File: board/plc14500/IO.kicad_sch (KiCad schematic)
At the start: 72 parts, among them U1 74HC14, U2 4051, U3 74HC14, U5 4099, U6 Arduino Nano

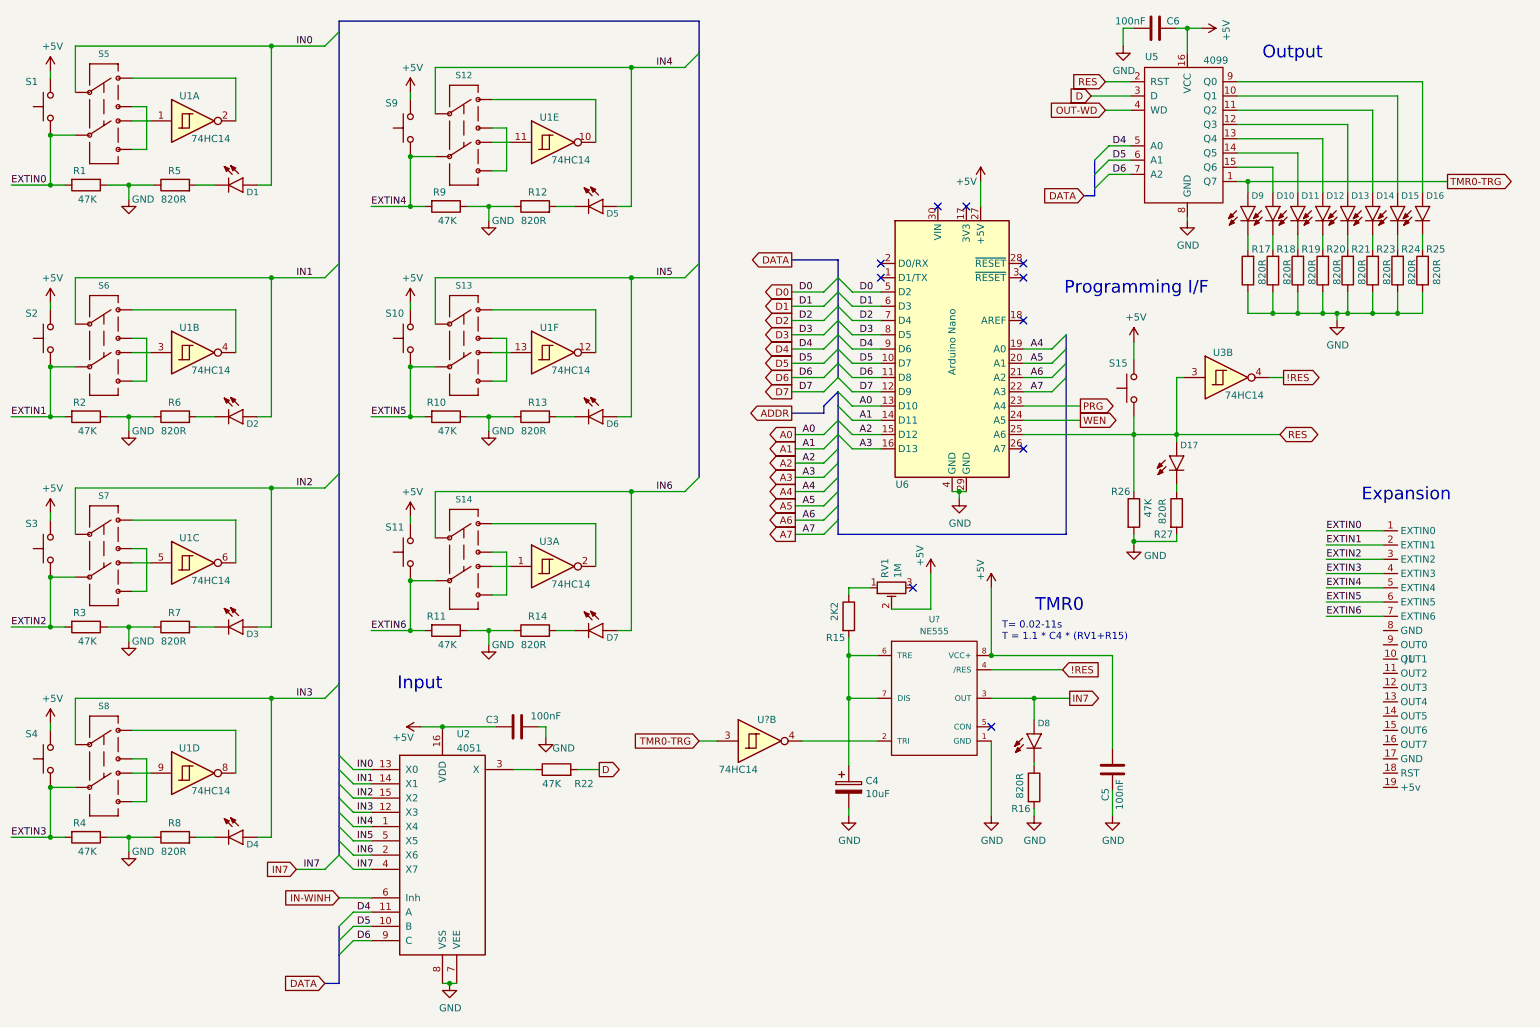
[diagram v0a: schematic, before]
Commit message: REV.D Schema updates
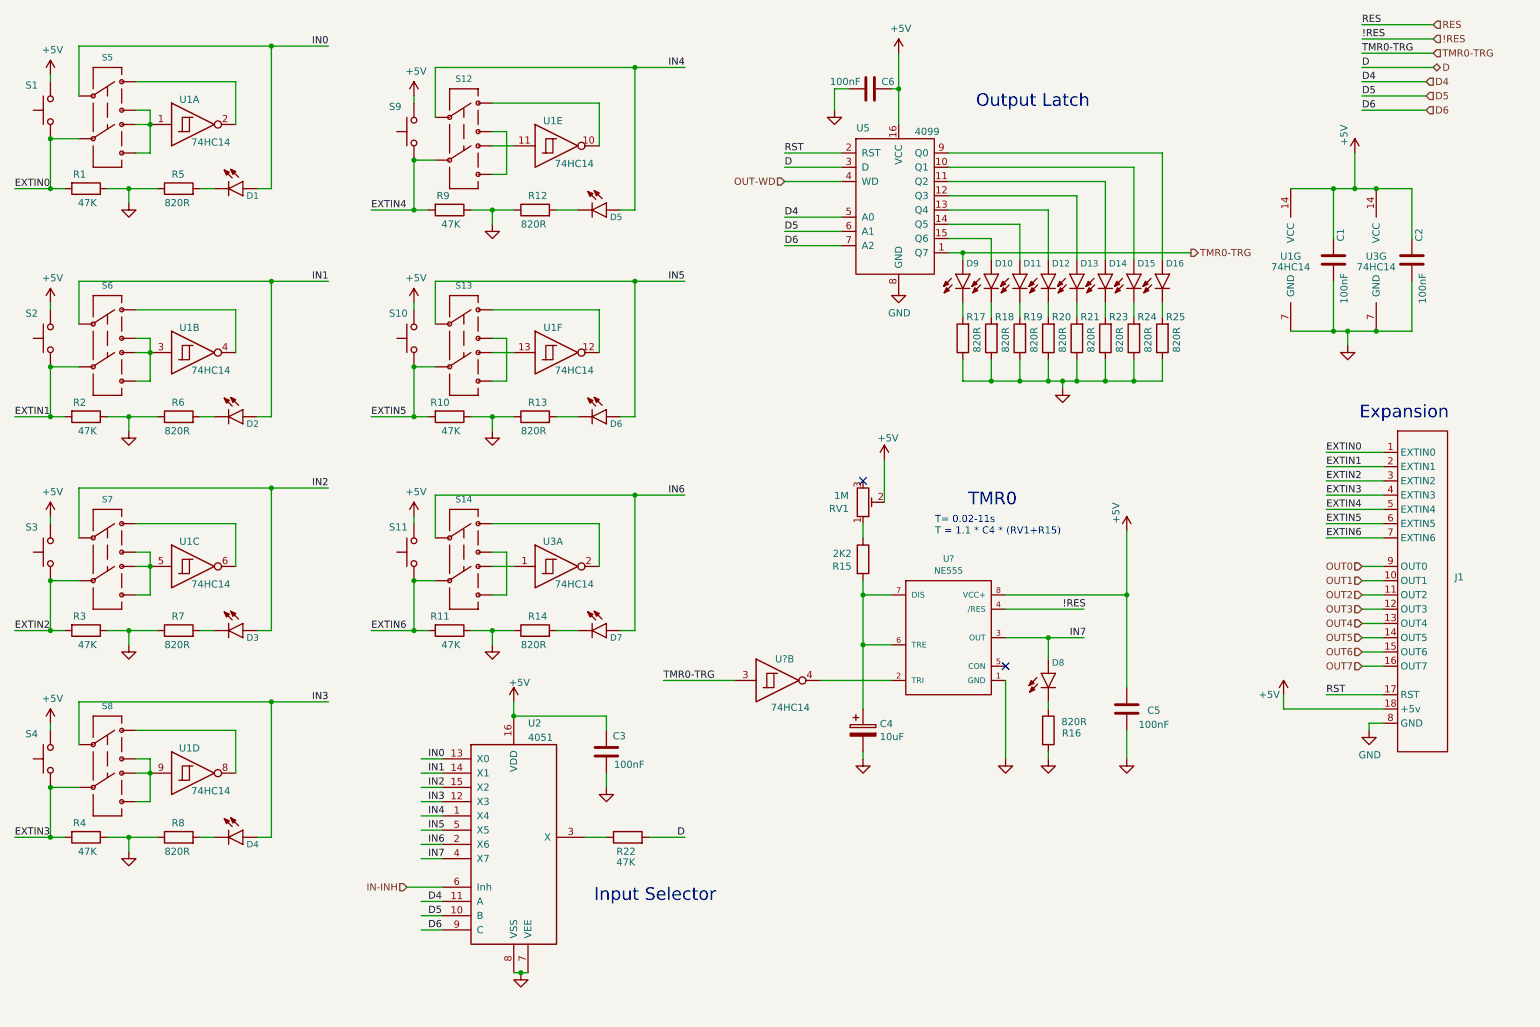
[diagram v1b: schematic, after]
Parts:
- removed D17: LED 3MM Red, plc14500:LED_3MM, symbol plc14500-rescue:LED5MM-SparkFun-LED
- removed R26: 47K, Resistor_THT:R_Axial_DIN0204_L3.6mm_D1.6mm_P7.62mm_Horizontal, symbol Device:R
- removed R27: 820R, Resistor_THT:R_Axial_DIN0204_L3.6mm_D1.6mm_P7.62mm_Horizontal, symbol Device:R
- removed S15: Push Button, plc14500:SW_Tactile_THT, symbol Switch:SW_Push
- removed unit 2 of U3
- removed U6: Arduino Nano, Module:Arduino_Nano, symbol MCU_Module:Arduino_Nano_v2.x
- added C1, C2: 100nF, Capacitor_THT:C_Rect_L7.2mm_W2.5mm_P5.00mm_FKS2_FKP2_MKS2_MKP2, symbol Device:C
- added unit 7 of U1
- added unit 7 of U3
- S12, S13, S14, S5, S6, S7, S8: symbol plc14500-rescue:SWITCH-DPDT-PTH-GPI-152-3013-SparkFun-Switches -> plc14500:SWITCH-DPDT
- U1, U3, U?: symbol 74xx:74HC14 -> plc14500:74HC14
- U?: symbol plc14500-rescue:555D-SparkFun-IC-Special-Function -> plc14500:555
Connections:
- net +5V: now also C3.1, J1.18 (+5v), C1.2, C2.2, U1.14 (VCC), U3.14 (VCC); no longer C3.2
- net GND: now also C3.2, J1.8 (GND), C1.1, C2.1, U1.7 (GND), U3.7 (GND); no longer C3.1
- net RES: no longer U5.2 (RST)
- net at S5.1: now also S5.5, S5.7, U1.1; no longer U1.2
- net at S5.3: now also U1.2; no longer S5.7
- net at S6.1: now also S6.5, S6.7, U1.3; no longer U1.4
- net at S6.3: now also U1.4; no longer S6.7
- net at S7.1: now also S7.5, S7.7, U1.5; no longer U1.6
- net at S7.3: now also U1.6; no longer S7.7
- net at S8.1: now also S8.5, S8.7, U1.9; no longer U1.8
- net at S8.3: now also U1.8; no longer S8.7
- net at S12.1: now also S12.5; no longer U1.10
- net at S12.3: now also U1.10; no longer S12.7
- net at U1.11: now also S12.7; no longer S12.5
- net at S13.1: now also S13.5; no longer U1.12
- net at S13.3: now also U1.12; no longer S13.7
- net at U1.13: now also S13.7; no longer S13.5
- net at S14.1: now also S14.5; no longer U3.2
- net at S14.3: now also U3.2; no longer S14.7
- net at U3.1: now also S14.7; no longer S14.5
- net OUT1: now reaches J1.10 (OUT1)
- net OUT2: now reaches J1.11 (OUT2)
- net OUT3: now reaches J1.12 (OUT3)
- net OUT4: now reaches J1.13 (OUT4)
- net OUT5: now reaches J1.14 (OUT5)
- net OUT6: now reaches J1.15 (OUT6)
- net OUT7: now reaches J1.16 (OUT7)
- net RST: now reaches J1.17 (RST)
- net RST: now also U5.2 (RST)
- net OUT0: now reaches J1.9 (OUT0)
- net IN-WINH renamed IN-INH
- no-connect marks 10 -> 2
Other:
- note added: "Input Selector"
- note added: "Output Latch"
- note removed: "Input"
- note removed: "Output"
- note removed: "Programming I/F"
- moved on the sheet: C3, C4, C5, C6, D1, D10, D11, D12, D13, D14, D15, D16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
